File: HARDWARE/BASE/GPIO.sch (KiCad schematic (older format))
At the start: 46 parts, among them U1201 SN74LVC1T45DBV, U1202 SN74LVC1T45DBV, U1203 SN74LVC1T45DBV, U1204 SN74LVC1T45DBV, U1205 SN74LVC1T45DBV, U1206 SN74LVC1T45DBV, U1207 SN74LVC1T45DBV, U1208 SN74LVC1T45DBV, U1209 SN74LVC1T45DBV, U1210 SN74LVC1T45DBV, U1211 SN74LVC1T45DBV, U1212 SN74LVC1T45DBV, U1213 SN74LVC1T45DBV, U1214 SN74LVC1T45DBV, U1215 MCP23S17_SO

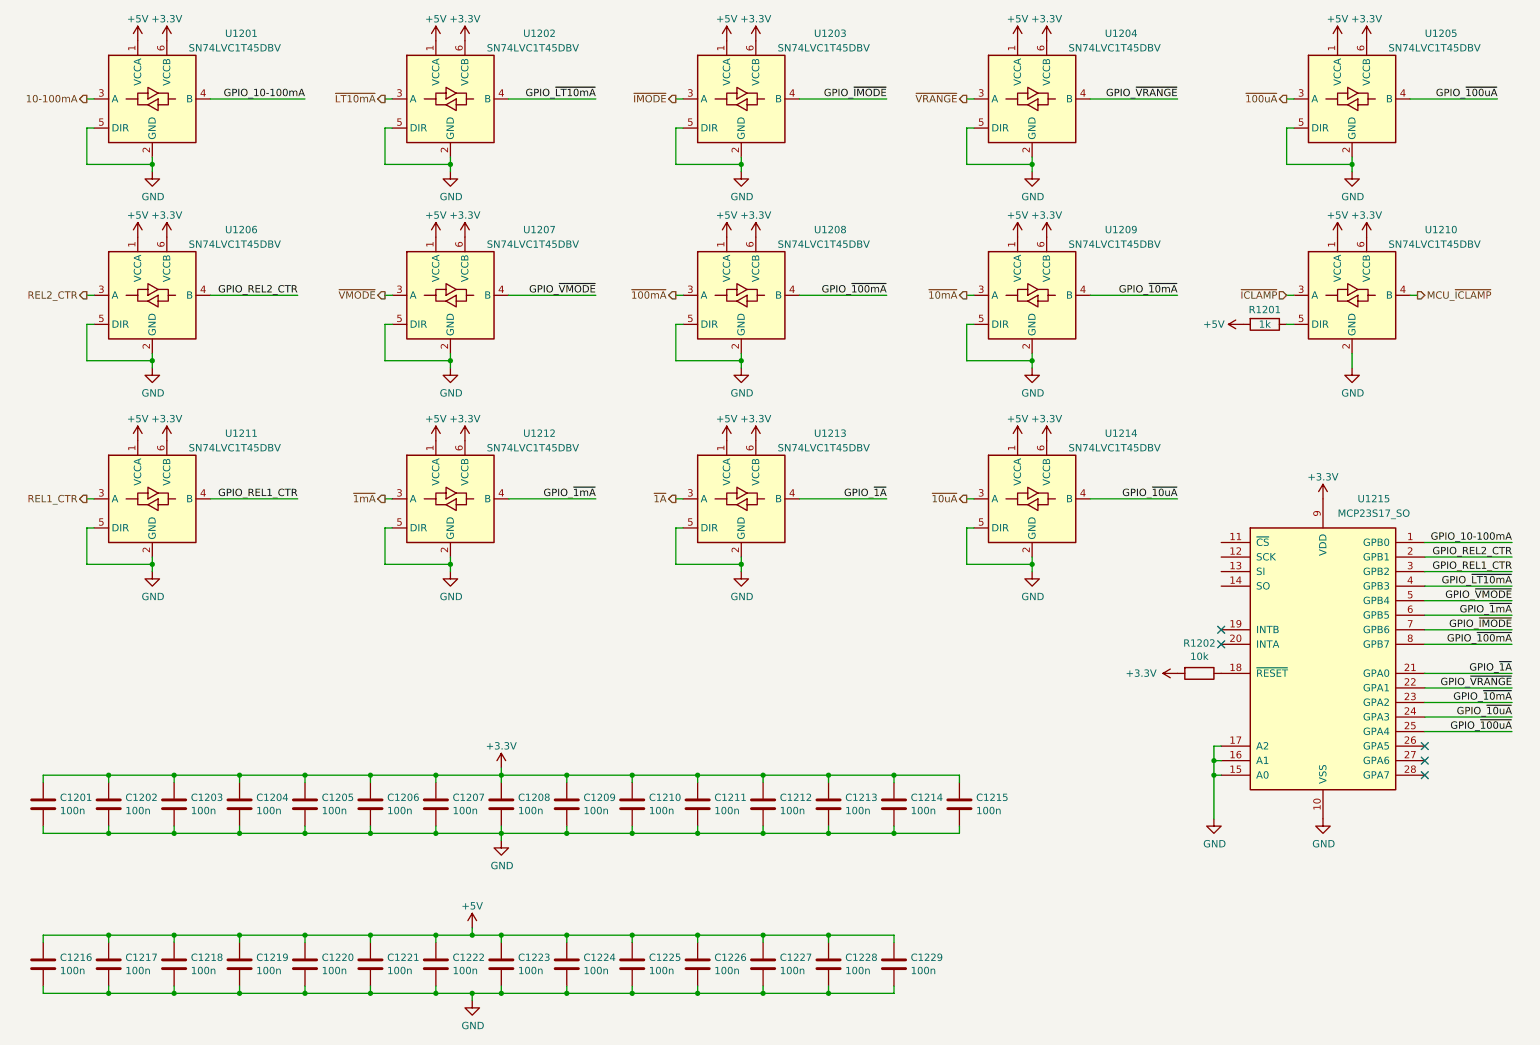
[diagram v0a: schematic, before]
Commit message: Schematic and PCB changes
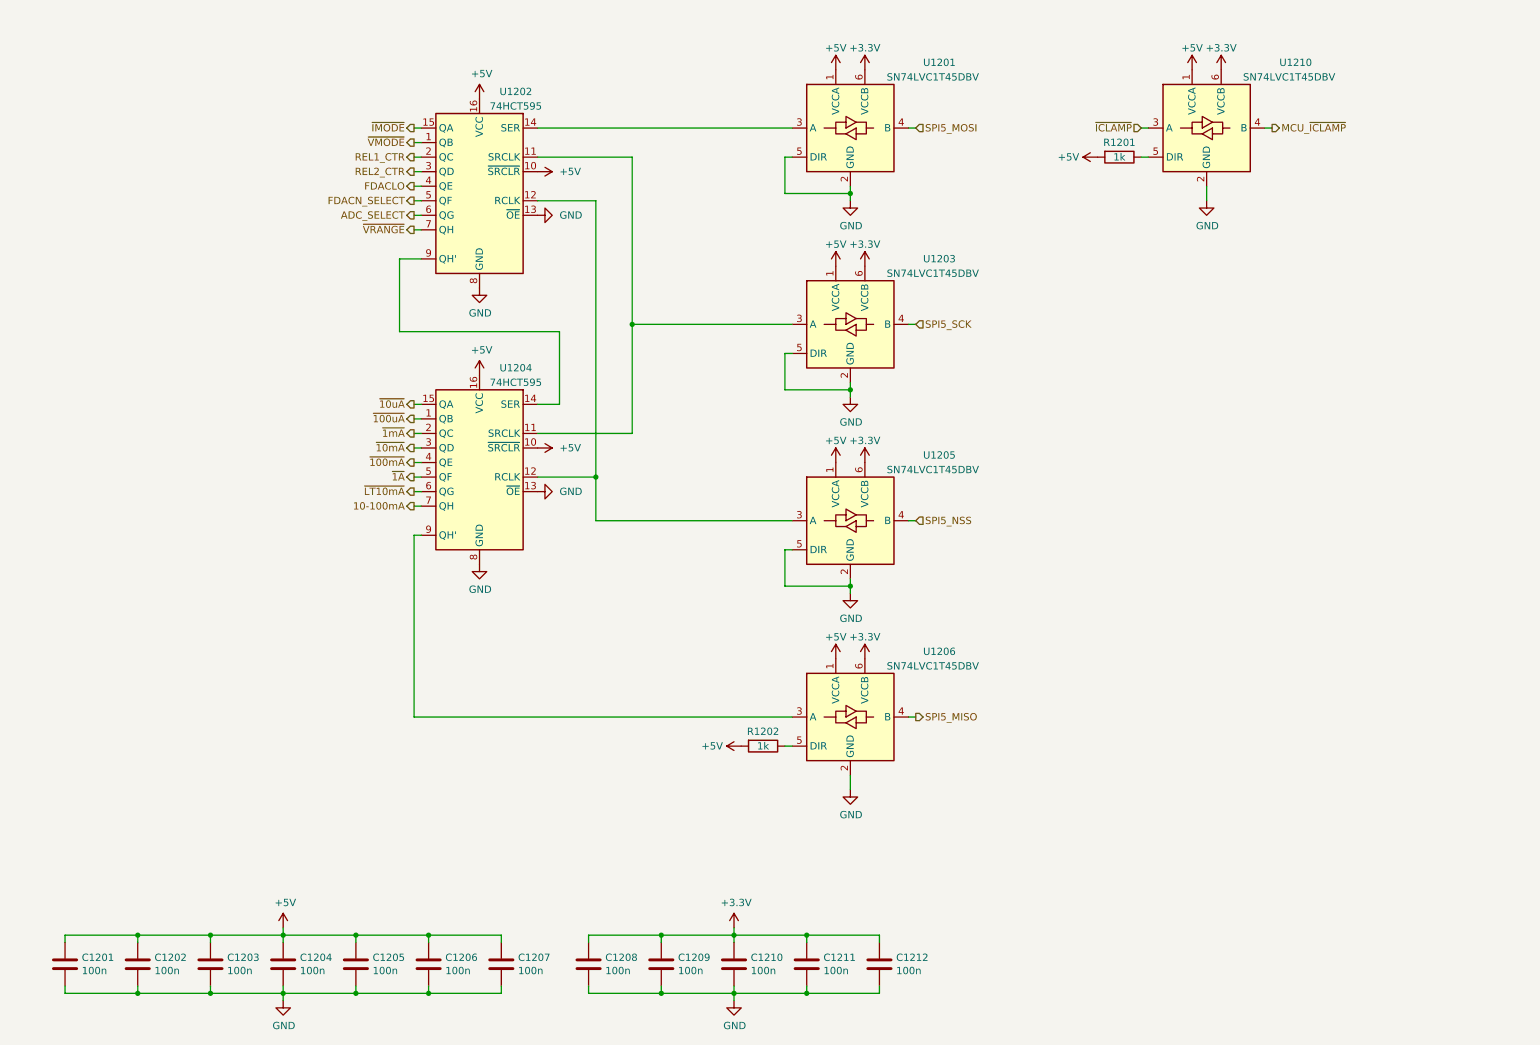
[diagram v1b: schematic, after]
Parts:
- removed C1213, C1214, C1215, C1216, C1217, C1218, C1219, C1220, C1221, C1222, C1223, C1224, C1225, C1226, C1227, C1228, C1229: 100n, Capacitor_SMD:C_0603_1608Metric_Pad1.08x0.95mm_HandSolder, symbol Device:C
- removed U1202, U1204, U1207, U1208, U1209, U1211, U1212, U1213, U1214: SN74LVC1T45DBV, Package_TO_SOT_SMD:SOT-23-6, symbol Logic_LevelTranslator:SN74LVC1T45DBV
- removed U1215: MCP23S17_SO, Package_SO:SOIC-28W_7.5x17.9mm_P1.27mm, symbol Interface_Expansion:MCP23S17_SO
- added U1202, U1204: 74HCT595, Package_SO:TSSOP-16_4.4x5mm_P0.65mm, symbol 74xx:74HCT595
- R1202: value 10k -> 1k
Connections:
- net +3V3: no longer C1201.1, C1202.1, C1203.1, C1204.1, C1205.1, C1206.1, C1207.1, R1202.2
- net +5V: now also C1201.1, C1202.1, C1203.1, C1204.1, C1205.1, C1206.1, C1207.1, R1202.2, U1202.10 (~SRCLR), U1202.16 (VCC), U1204.10 (~SRCLR), U1204.16 (VCC)
- net 10-100mA: now also U1204.7 (QH); no longer U1201.3 (A)
- net GND: now also U1202.13 (~OE), U1202.8 (GND), U1204.13 (~OE), U1204.8 (GND); no longer U1206.5 (DIR)
- net REL1_CTR: now also U1202.2 (QC)
- net REL2_CTR: now also U1202.3 (QD); no longer U1206.3 (A)
- net ~100mA: now also U1204.4 (QE)
- net ~100uA: now also U1204.1 (QB); no longer U1205.3 (A)
- net ~10mA: now also U1204.3 (QD)
- net ~10uA: now also U1204.15 (QA)
- net ~1A: now also U1204.5 (QF)
- net ~1mA: now also U1204.2 (QC)
- net ~IMODE: now also U1202.15 (QA); no longer U1203.3 (A)
- net ~LT10mA: now also U1204.6 (QG)
- net ~VMODE: now also U1202.1 (QB)
- net ~VRANGE: now also U1202.7 (QH)
- net at R1202.1: now also U1206.5 (DIR)
- net GPIO_10-100mA renamed SPI5_MOSI
- net GPIO_REL2_CTR renamed SPI5_MISO
- net GPIO_~100uA renamed SPI5_NSS
- net GPIO_~IMODE renamed SPI5_SCK
- new net: U1202.11 (SRCLK), U1203.3 (A), U1204.11 (SRCLK)
- new net: U1202.12 (RCLK), U1204.12 (RCLK), U1205.3 (A)
- new net: U1201.3 (A), U1202.14 (SER)
- new net: U1202.9 (QH'), U1204.14 (SER)
- new net: U1204.9 (QH'), U1206.3 (A)
- new net ADC_SELECT: U1202.6 (QG)
- new net FDACLO: U1202.4 (QE)
- new net FDACN_SELECT: U1202.5 (QF)
- no-connect marks 5 -> 0
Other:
- moved on the sheet: R1201, U1210
